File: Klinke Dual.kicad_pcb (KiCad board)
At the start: 2 copper layers, 30 x 30 mm, 9 parts, among them J1 AudioJack3_Dual_Ground_Switch, J2 Conn_01x03, J3 Conn_01x03

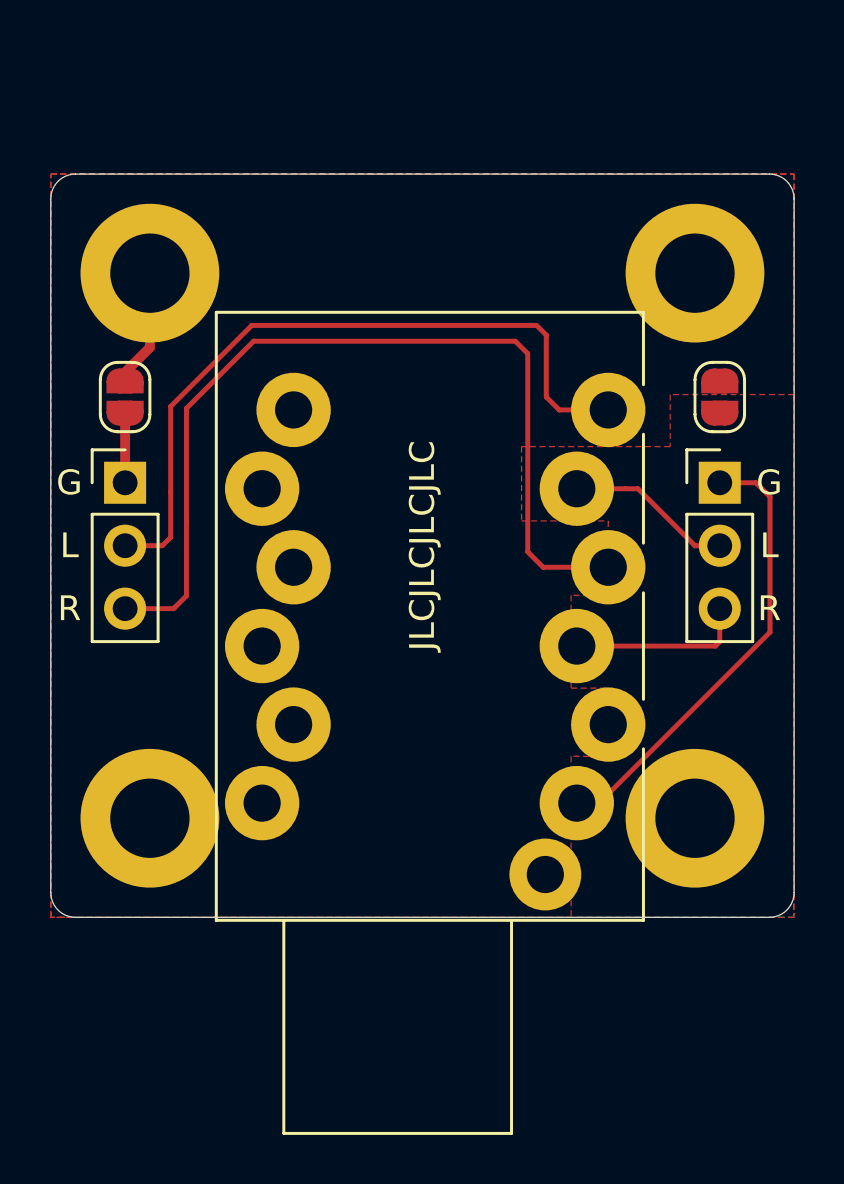
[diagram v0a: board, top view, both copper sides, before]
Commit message: Update to latest files
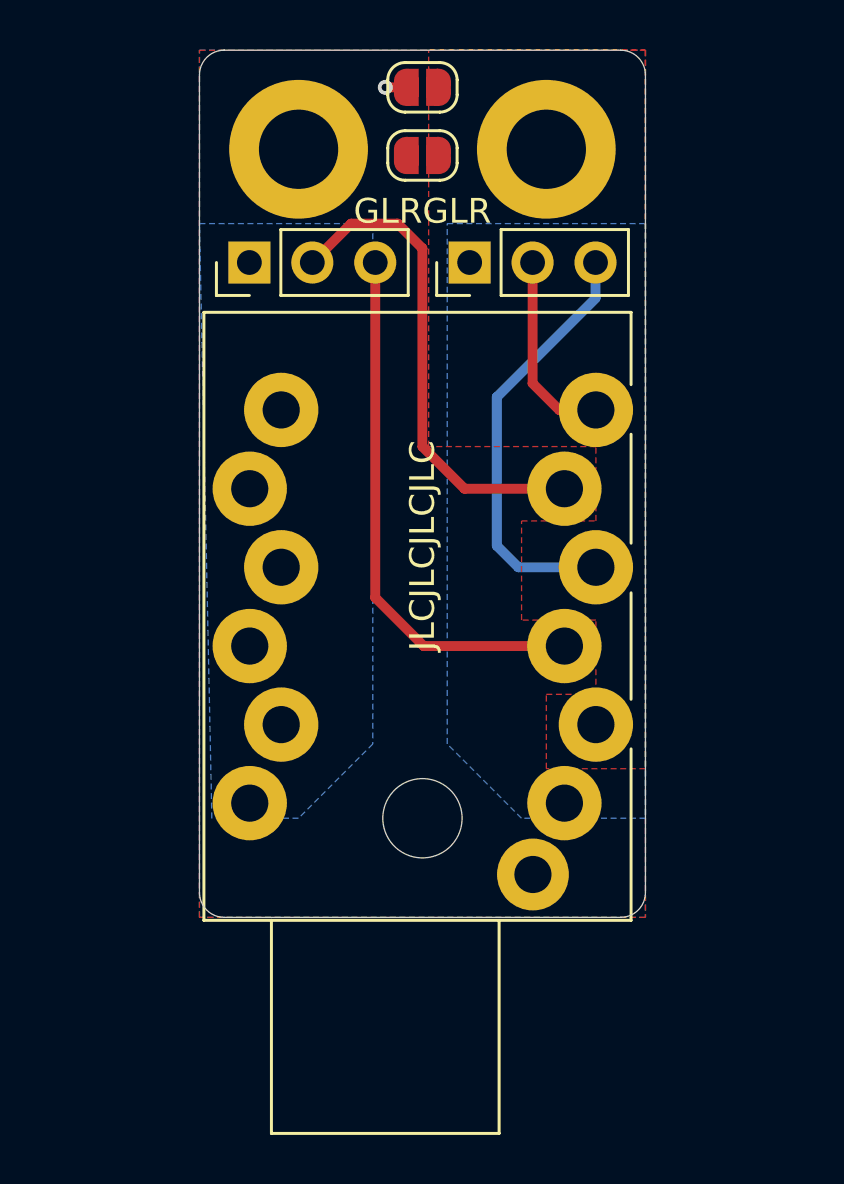
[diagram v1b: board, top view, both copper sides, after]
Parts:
- removed H4: MountingHole_Pad, MountingHole:MountingHole_3.2mm_M3_DIN965_Pad
- H3: value MountingHole_Pad -> MountingHole; footprint MountingHole:MountingHole_3.2mm_M3_DIN965_Pad -> MountingHole:MountingHole_3.2mm_M3_DIN965
- moved J3 21.0 mm to (143.0, 88.6), turned to 90 degrees
- moved JP1 17.3 mm to (150.0, 81.5), turned to 180 degrees
- moved J2 16.5 mm to (151.9, 88.6), turned to 90 degrees
- moved JP2 15.5 mm to (150.0, 84.2), turned to 180 degrees
- moved H3 11.0 mm to (150.0, 111.0)
- moved H1 7.81 mm to (145.0, 84.0)
- moved H2 7.81 mm to (155.0, 84.0)
- moved J1 0.50 mm to (157.0, 94.5)
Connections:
- H3 pad 1: Earth -> (no net)
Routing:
- net /LEFT1: track 29.2 -> 7.88 mm
- net /RIGHT1: track 36.9 -> 17.4 mm
- net /GND2: track 18.4 -> 0.00 mm
- net /RIGHT2: track 7.18 -> 22.0 mm
- net /LEFT2: track 6.72 -> 19.9 mm
- net Earth: track 4.76 -> 0.85 mm, vias 0 -> 1
- net /GND1: track 2.46 -> 0.00 mm
- added copper zone on B.Cu, net /GND1
- added copper zone on B.Cu, net /GND2
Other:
- board size 30 x 30 mm -> 18 x 35 mm
- board text added: "Dual Klinke Rev. 2, 2021-03-13 Tobias Müller, twam.info"
- board text added: "GLRGLR"
- board text removed: "Dual Klinke Rev. 1, 2021-03-06 Tobias Müller, twam.info"
- board text removed: "G"
- board text removed: "L"
- board text removed: "R"
